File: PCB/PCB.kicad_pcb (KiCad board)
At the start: 2 copper layers, 21 x 51 mm, 33 parts, among them J1 USB_C_Receptacle_USB2.0_16P, J2 Conn_01x20, J3 Conn_01x20, SW1 SW_Push, U1 RP2040, U2 MCP1700x-330xxTT, U3 W25Q128JVS, Y1 Crystal_GND24

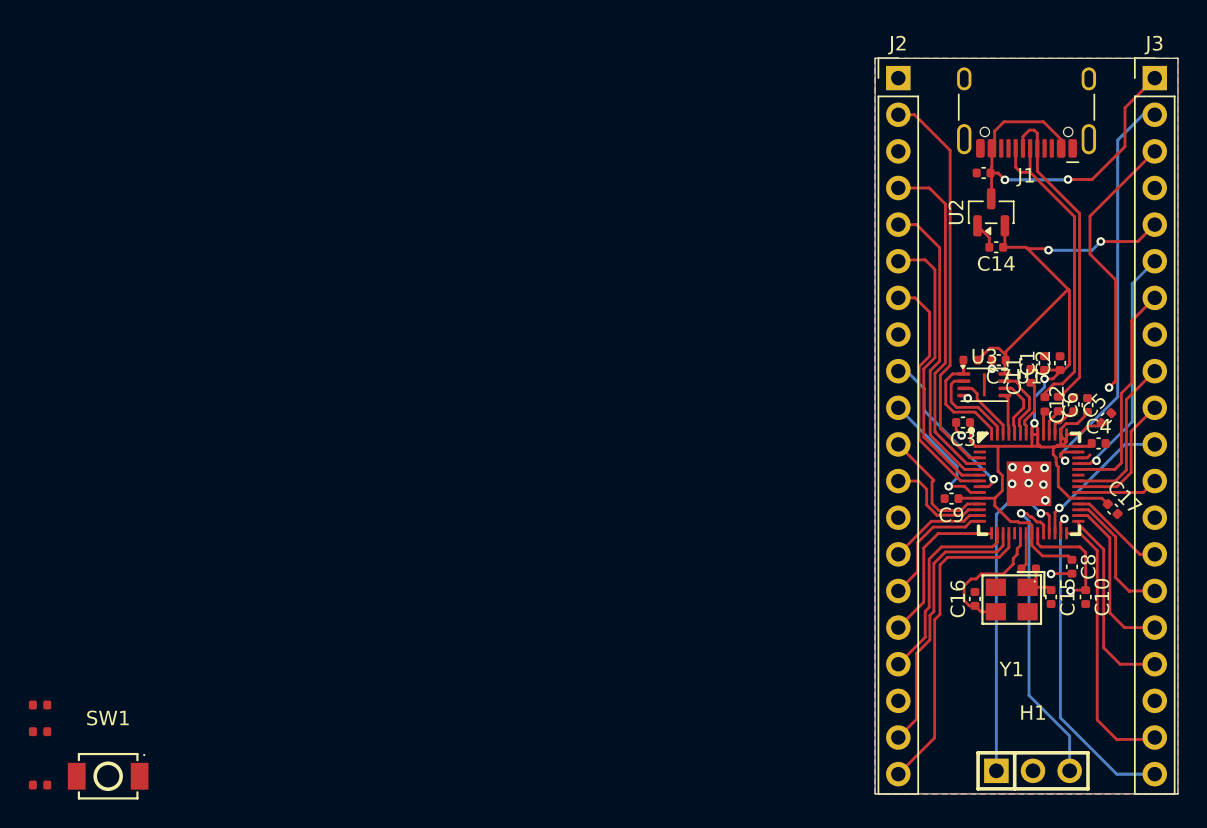
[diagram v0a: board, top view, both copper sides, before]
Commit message: Done with PCB, working on Silkscreen
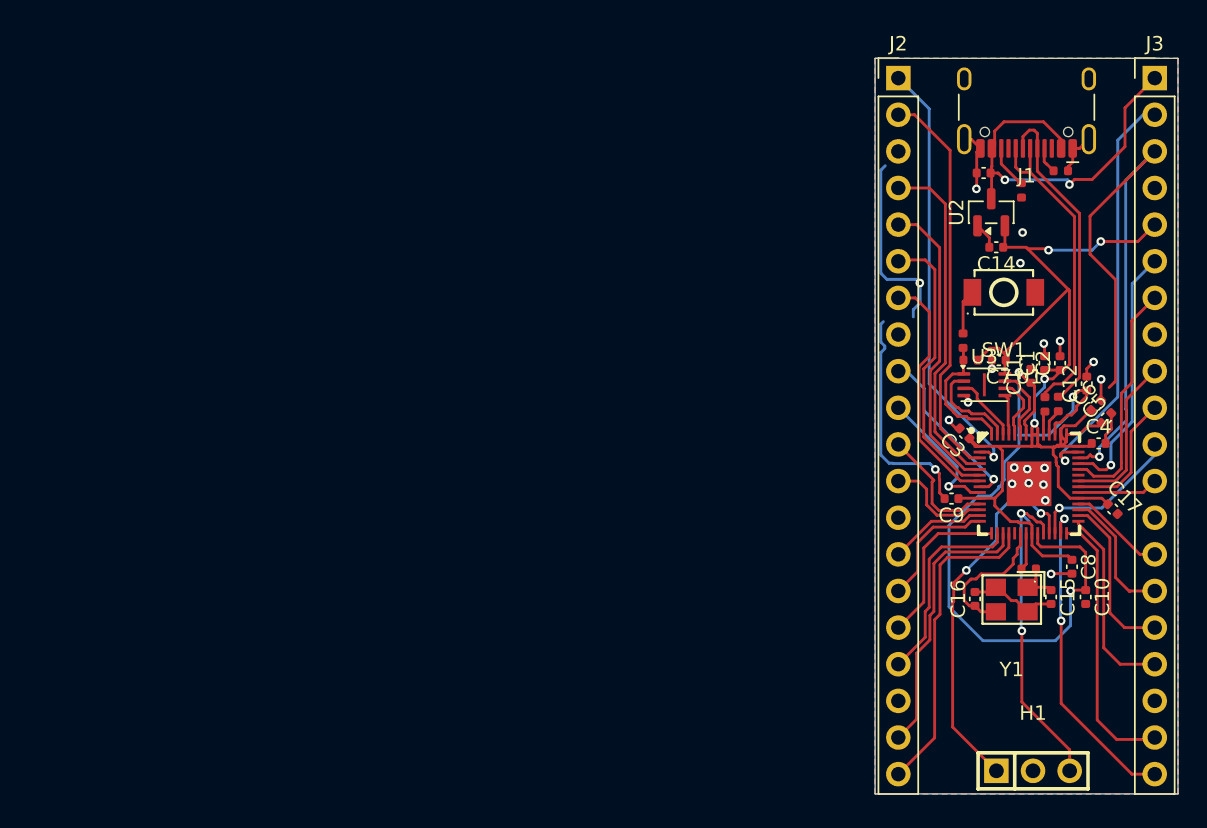
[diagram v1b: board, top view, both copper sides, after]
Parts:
- moved R2 80.7 mm to (134.3, 45.0)
- moved R1 76.8 mm to (131.6, 46.4), turned to -90 degrees
- moved R4 71.0 mm to (127.5, 56.8), turned to -90 degrees
- moved SW1 70.6 mm to (130.4, 53.5), turned to 180 degrees
- moved C12 1.70 mm to (136.1, 59.8)
- moved C3 0.76 mm to (127.7, 63.2), turned to 135 degrees
- moved C6 0.60 mm to (136.8, 61.3), turned to 45 degrees
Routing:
- net GND: track 5.36 -> 55.3 mm, vias 11 -> 20
- net +1V1: track 14.1 -> 55.1 mm, vias 1 -> 3
- net /GPIO0: track 0.00 -> 30.1 mm, vias 0 -> 1
- net /GPIO28: track 20.1 -> 43.6 mm
- net Net-(R4-Pad1): track 0.00 -> 3.12 mm
- net Net-(J1-CC2): track 0.00 -> 3.03 mm
- net /SWD: track 24.0 -> 26.5 mm, vias 1 -> 2
- net Net-(J1-CC1): track 0.00 -> 1.85 mm
- net /GPIO27: track 16.8 -> 18.0 mm
- net /QSPI_SS: track 8.32 -> 9.20 mm
- net /SWCLK: track 21.7 -> 22.5 mm, vias 1 -> 2
- net /GPIO26: track 15.6 -> 16.2 mm
- net /GPIO16: track 23.2 -> 22.6 mm, vias 1 -> 2
- added copper zone on In1.Cu, net GND
- added copper zone on In2.Cu, net GND
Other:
- copper layers 2 -> 4
